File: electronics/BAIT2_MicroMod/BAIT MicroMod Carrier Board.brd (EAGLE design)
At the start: 95.2 x 94 mm, 108 parts, among them J1 microSD, J4 JST_6_PIN_VERTICAL, J5 QWIIC_RIGHT_ANGLE, U3 3.3V, U4 3.3V, U5 BQ27441-G1, X1 2.1mm DC, X2 BQ24074

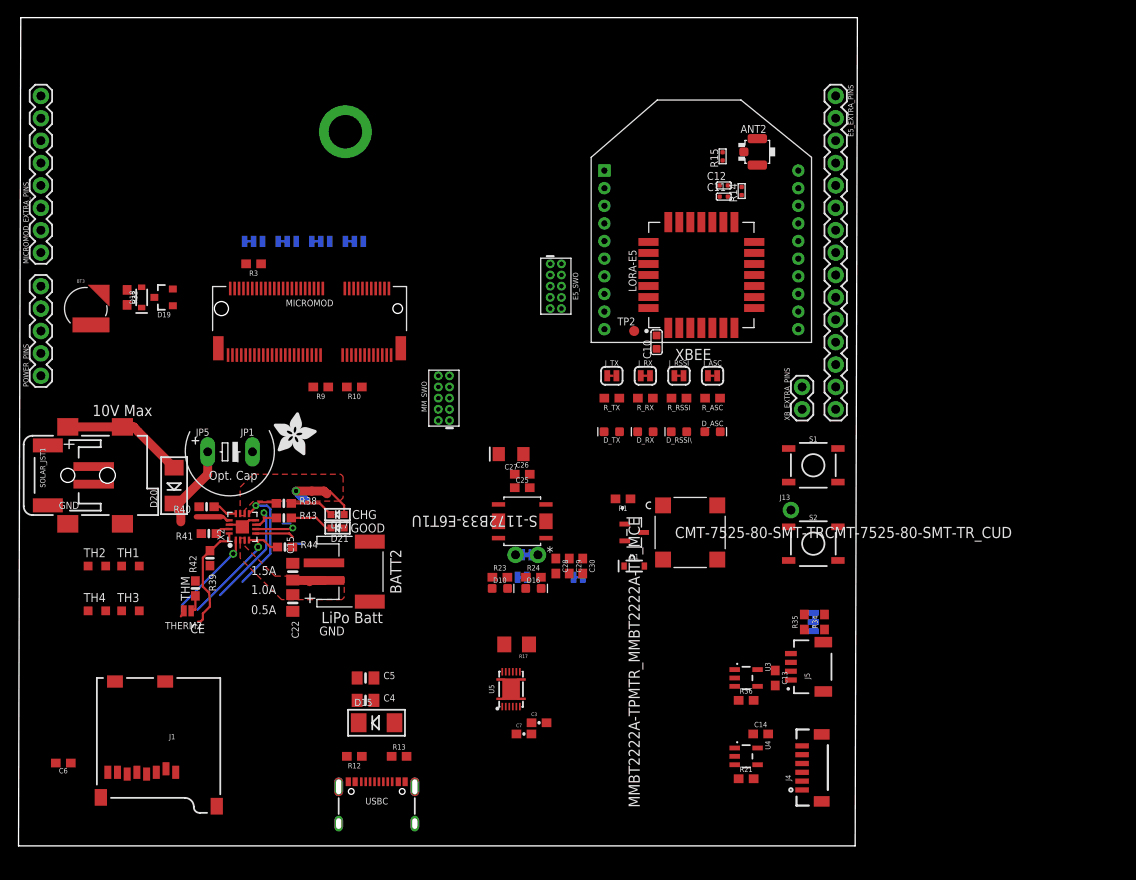
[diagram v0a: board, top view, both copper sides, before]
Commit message: Files for First Prototype production
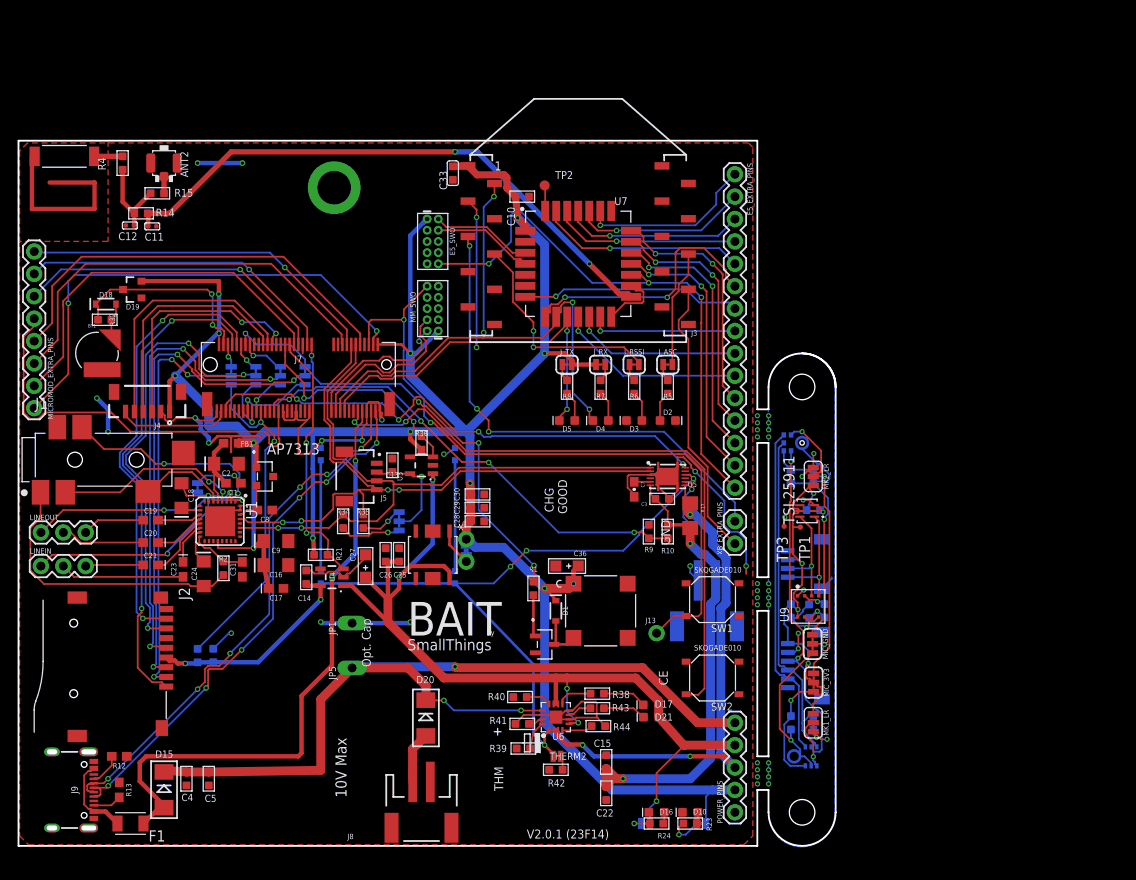
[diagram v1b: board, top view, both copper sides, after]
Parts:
- removed 3V3_LED2: (no value), SparkFun-Jumpers:SMT-JUMPER_2_NC_TRACE_SILK
- removed BATT2: JST 2PH, adafruit:JST-PH-2-SMT-RA
- removed BT3: ML414H, SparkFun-Batteries:ML414H_IV01E
- removed D_ASC, D_RSSI\, D_RX: GREEN, SparkFun-LED:LED-0603
- removed D_TX: RED, SparkFun-LED:LED-0603
- removed LORA-E5: LoRa-E5-HF, moudle-new:MOUDLE28P-1.25-12X12X2.5MM
- removed MICROMOD: MICROMOD-2222-C, SparkFun-MicroMod:M.2-CONNECTOR-E
- removed REG1: S-1172B33-E6T1U, Ablic:HSOP-6_FH006-A-P-SD-2.1_ABL
- removed R_ASC: 4.7k, SparkFun-Resistors:0603
- removed R_RSSI, R_RX, R_TX: 1k, SparkFun-Resistors:0603
- removed S1: Reset, SparkFun-Switches:TACTILE_SWITCH_SMD_5.2MM
- removed S2: BOOT, SparkFun-Switches:TACTILE_SWITCH_SMD_5.2MM
- removed SOLAR_JST1: (no value), SparkFun-Connectors:JST-2-SMD
- removed U$23: (no value), microbuilder:ADAFRUIT_5MM
- removed USBC: (no value), SparkFun-Connectors:USB-C-16P-2LAYER-PADS
- removed X1: 2.1mm DC, microbuilder:DCJACK_2MM_SMT
- removed X2: BQ24074, adafruit_power:QFN16_3MM
- removed XBEE: XBEE, adafruit:XBEE
- added 3V3_LED, GND_CON: (no value), SparkFun-Jumpers:SMT-JUMPER_2_NC_TRACE_SILK
- added ANT1: 0868AT43A0020EANT_0868AT43A0020E_JOT, 2023-01-04_20-35-52_Library:ANT_0868AT43A0020E_JOT
- added BT1: ML414H, SparkFun-Batteries:ML414H_IV01E
- added C1, C17, C19, C20, C21, C23, C31, C8: 2.2uF, SparkFun-Capacitors:0603-POLAR
- added C16, C2, C24, C9: 0.1uF, SparkFun-Capacitors:EIA3216
- added C18: 0.15uF, SparkFun-Capacitors:EIA3216
- added C32, C34, C35, C37, C38: 100nf, OPL_Capacitor:C0603
- added C33: 4.7uF, Discrete-new:C0603
- added C36: 10uf, OPL_Capacitor:AVX-A
- added C39: 220pF, Capacitor:CAPC1608X85
- added D2, D3, D4: GREEN, SparkFun-LED:LED-0603
- added D5: RED, SparkFun-LED:LED-0603
- added F1: 6V/2A, Circuit-Protection:FUSC3215X82N
- added FB1: 600Ω/1.8A, SparkFun-Coils:0603
- added J10: QWIIC_RIGHT_ANGLE, SM04B-SRSS-TB_LF__SN_:JST_SM04B-SRSS-TB(LF)(SN)
- added J15: SM06B-SRSS-TB(LF)(SN), SM06B-SRSS-TB_LF__SN_:JST_SM06B-SRSS-TB(LF)(SN)
- added J2: ST-TF-003A, ST-TF-003A:SUNTECH_ST-TF-003A
- added J3: (no value), SparkFun-RF:XBEE-SMD
- added J6: JST 2PH, adafruit:JST-PH-2-SMT-RA
- added J7: MICROMOD-2222-C, SparkFun-MicroMod:M.2-CONNECTOR-E
- added J8: (no value), SparkFun-Connectors:JST-2-SMD
- added J9: (no value), SparkFun-Connectors:USB-C-16P-2LAYER-PADS
- added LINEIN, LINEOUT: (no value), SparkFun-Connectors:1X03
- added MIC_3V3, MIC_GND: (no value), SparkFun-Jumpers:SMT-JUMPER_3_2-NC_TRACE_SILK
- added MK1: ICS-43432, Audio-Devices:ICS-43432
- added MK1_LR: MK1_LR, SparkFun-Jumpers:SMT-JUMPER_3_1-NC_TRACE_SILK
- added MK2: SPH0645LM4H-B, SPH0645LM4H-B:MIC_SPH0645LM4H-B
- added MK2_LR: MK2_LR, SparkFun-Jumpers:SMT-JUMPER_3_1-NC_TRACE_SILK
- added R11, R5: 4.7K, OPL_Resistor:R0603
- added R18: 100K, OPL_Resistor:R0603
- added R2: 2.2K, OPL_Resistor:R0603
- added R4: 0R, OPL_Resistor:R0603
- added R6, R7, R8: 1K 1/10W, OPL_Resistor:R0603
- added SW1, SW2: SKQGADE010, OPL_Switch:SW4-SMD-5.2X5.2X1.5MM
- added TP1, TP3: PTR1TP06R, testpad:TP06R
- added U1: SGTL5000-32, Freescale:QFN-32-5MM
- added U10: TSL25911, 2023-02-07_20-42-29_Library:SON-06-FN_2000X2400_AMS
- added U2: AP7313, 2022-08-05_10-01-44_Library:SOT-23_DIO
- added U6: BQ24074, adafruit_power:QFN16_3MM
- added U7: LoRa-E5-HF, moudle-new:MOUDLE28P-1.25-12X12X2.5MM
- added U8: S-1172B33-E6T1U, Ablic:HSOP-6_FH006-A-P-SD-2.1_ABL
- added U9: BOSCH_TOOLS_BME680BOSCH_TOOLS_BME680_0_0, Bosch Tools - BME680:BOSCH_TOOLS_BME680_0
- C10: value 4.7uF -> 4.7uf; device Discrete-new:C0603 -> OPL_Capacitor:C0603
- C13, C14, C28: value 1.0uF -> 1uf; device SparkFun-Capacitors:0603 -> OPL_Capacitor:C0603
- C15, C22, C4, C5: value 10uF -> 4.7uf; device microbuilder:0805-NO -> OPL_Capacitor:C0603
- C25, C30: value 0.22uF -> 220nf; device SparkFun-Capacitors:0603 -> OPL_Capacitor:C0603
- C26, C29, C6: value 0.1uF -> 100nf; device SparkFun-Capacitors:0603 -> OPL_Capacitor:C0603
- C27: value 10uF -> 10uf; device SparkFun-Capacitors:EIA3216 -> OPL_Capacitor:AVX-A
- C3: value 1.0uF -> 1uf; device SparkFun-Capacitors:0603-CAP -> OPL_Capacitor:C0603
- D17, D21: device microbuilder:CHIPLED_0603 -> SparkFun-LED:LED-0603
- J1: value microSD -> SJ-43516-SMT; device SparkFun-Connectors:MICRO-SD-SOCKET -> SnapEDA-Library:CUI_SJ-43516-SMT
- R1: value 180 -> 200K; device SparkFun-Resistors:0603 -> OPL_Resistor:R0603
- R10: value 20k -> 20K; device SparkFun-Resistors:0603 -> OPL_Resistor:R0603
- R14, R15: device Discrete-new:R0402 -> OPL_Resistor:R0603
- R21, R3, R36: value 100k -> 100K; device SparkFun-Resistors:0603 -> OPL_Resistor:R0603
- R23: value 1k -> 1K 1/10W; device SparkFun-Resistors:0603 -> OPL_Resistor:R0603
- R24: value 4.7k -> 4.7K; device SparkFun-Resistors:0603 -> OPL_Resistor:R0603
- R32: value 3.3k -> 3.3K; device SparkFun-Resistors:0603 -> OPL_Resistor:R0603
- R34, R35: value 2.2k -> 2.2K; device SparkFun-Resistors:0603 -> OPL_Resistor:R0603
- R38, R41, R42, R43, R44: value 10K -> 10K 1/10W; device microbuilder:0603-NO -> OPL_Resistor:R0603
- R39: device microbuilder:0603-NO -> OPL_Resistor:R0603
- R40: value 1K -> 1K 1/10W; device microbuilder:0603-NO -> OPL_Resistor:R0603
- R9: value 10k -> 10K 1/10W; device SparkFun-Resistors:0603 -> OPL_Resistor:R0603
- TH1, TH2, TH3, TH4: device varistor:CT/CN0603 -> NTCG163JX103DT1S:THERM_NTCG163JX103DT1S
- moved POWER_PINS 93.0 mm to (81.3, 3.81)
- moved J4 86.3 mm to (14.6, 50.5), turned to 180 degrees
- moved R14 68.2 mm to (13.9, 71.8), turned to 270 degrees
- moved C12 67.5 mm to (12.6, 70.4)
- moved ANT2 67.3 mm to (16.5, 77.5), turned to 90 degrees
- moved C11 64.9 mm to (15.2, 70.3), turned to 180 degrees
- moved R15 64.3 mm to (15.7, 74.0)
- moved R34 55.8 mm to (36.8, 36.8), turned to 0 degrees
- moved C14 54.5 mm to (32.6, 30.5), turned to 180 degrees
- moved R21 54.5 mm to (34.3, 33.0), turned to 270 degrees
- moved J5 51.7 mm to (40.6, 41.9), turned to 270 degrees
- moved R35 51.3 mm to (39.1, 36.8), turned to 0 degrees
- moved U4 51.2 mm to (35.6, 30.5), turned to 90 degrees
- moved C13 49.7 mm to (42.4, 43.2), turned to 180 degrees
- moved QWIIC_PWR 48.4 mm to (43.2, 36.8)
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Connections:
- removed net GND1: SOLAR_JST1.1, X1.2, X1.3
- removed net OUT: X2.5
- removed net PA15/SDA: LORA-E5.6
- removed net PB15/SCL: LORA-E5.5
- removed net RX2: MICROMOD.20
- removed net THERM: TH1.1, TH3.1, THERM2.2, X2.1
- removed net TX2: MICROMOD.22
- removed net V+1: REG1.6
- removed net VCC: XBEE.1
- new net 3V3_B: C34.1, C35.1, J10.2, J15.1, MIC_3V3.2, MK1_LR.1, MK2_LR.3, TP1.TP, U10.5, U9.8
- new net 3V3_ICS: C37.1, MIC_3V3.3, MK1.3
- new net 3V3_SPH: C38.1, C39.1, MIC_3V3.1, MK2.5
- new net AGND: C18.-, GND_CON.1, LINEIN.1, LINEOUT.1, U1.1, U1.3, U1.7
- new net GND_B: C32.2, C34.2, C35.2, J10.1, J10.S1, J10.S2, J15.2, J15.S1, J15.S2, MIC_GND.2, MK1_LR.3, MK2_LR.1, R18.1, TP3.TP, U10.3, U9.1, U9.5, U9.7
- new net GND_ICS: C37.2, MIC_GND.3, MK1.2, MK1.4
- new net GND_SPH: C38.2, C39.2, MIC_GND.1, MK2.3
- new net INT_B: U10.2
- new net N$11: ANT1.1, R4.2
- new net N$13: C19.-, LINEOUT.3
- new net N$14: C20.-, LINEOUT.2
- new net N$15: C21.-, LINEIN.3
- new net N$17: C23.-, LINEIN.2
- new net N$18: C19.+, U1.11
- new net N$20: C20.+, U1.12
- new net N$21: C21.+, U1.13
- new net N$22: C23.+, U1.14
- new net N$33: C24.-, J1.1, R2.2
- new net N$35: J1.3, U1.2
- new net N$36: F1.1, J9.VBUS1, J9.VBUS2
- new net N$38: C18.+, U1.10
- new net N$39: C31.+, R2.1, U1.16
- new net N$40: C24.+, U1.15
- new net N$41: C8.+, U1.30, U2.2
- new net N$46: C1.+, C2.+, FB1.2, U1.5
- new net N$54: C32.1, R11.2, U9.6
- new net N$55: R11.1, U9.2
- new net N$8: J1.2, U1.6
- new net SCK_B: J15.3, MK1.6, MK2.4
- new net SCL_B: J10.4, U10.1, U9.4
- new net SDA_B: J10.3, U10.6, U9.3
- new net SD_B: J15.4, MK1.7, MK2.6, R18.2
- new net SEL_MK1: MK1.1, MK1_LR.2
- new net SEL_MK2: MK2.2, MK2_LR.2
- new net USB_VIN: D15.A, F1.2, J7.9
- new net WS_B: J15.5, MK1.5, MK2.1
- net !BOOT!: now also J7.11, SW2.2; no longer MICROMOD.11, S2.3, S2.4
- net !CE: now also U6.4; no longer X2.4
- net !CHG: now also U6.9; no longer X2.9
- net !PGOOD: now also U6.7; no longer X2.7
- net !RESET!: now also J7.6, SW1.2; no longer MICROMOD.6, S1.3, S1.4
- net 3.3V: now also 3V3_LED.2, C16.+, C17.+, C33.2, C36.+, C9.+, FB1.1, J3.1, J7.2, J7.74, J_RX.1, U1.20, U2.1, U7.1; no longer 3V3_LED2.2, J_RX.2, LORA-E5.1, MICROMOD.2, MICROMOD.74
- net 3.3V_EN: now also J7.4; no longer MICROMOD.4
- net 3.3V_LP: now also J2.4; no longer J1.VCC
- net A0: now also J7.34; no longer MICROMOD.34
- net A1: now also J7.38; no longer MICROMOD.38
- net ASC: now also J3.15; no longer XBEE.15
- net CLK/SCK: now also J2.5, JP_SCK.2; no longer J1.SCLK, JP_SCK.3
- net CMD/CIPO: now also J2.3, JP_CIPO.2; no longer J1.DI/CMD, JP_CIPO.3
- net D0: now also J7.10; no longer MICROMOD.10
- net D1: now also J7.18; no longer MICROMOD.18
- net DAT0/COPI: now also J2.7, JP_COPI.2; no longer J1.DO/DAT0, JP_COPI.3
- net DAT3/!CS!: now also J2.2, JP_CS.2; no longer J1.CS/DAT3, JP_CS.3
- net GND: now also BT1.-, C1.-, C16.-, C17.-, C2.-, C31.-, C33.1, C36.-, C8.-, C9.-, D2.C, D3.C, GND_CON.2, J2.6, J2.G1, J2.G2, J2.G3, J2.G4, J3.10, J6.2, J7.1, J7.33, J7.36, J7.39, J7.45, J7.7, J7.75, J8.1, J9.GND, J9.GND2, SW1.4, SW2.4, U1.31, U1.32, U1.PAD, U2.3, U6.14, U6.6, U6.8, U6.THERMAL, U7.14, U7.16, U7.2, U7.22, U8.2, U8.5; no longer BATT2.2, BT3.-, D_ASC.C, D_RSSI\.C, J1.CD1, J1.GND, J1.GND1, J1.GND3, LORA-E5.14, LORA-E5.16, LORA-E5.2, LORA-E5.22, MICROMOD.1, MICROMOD.33, MICROMOD.36, MICROMOD.39, MICROMOD.45, MICROMOD.7, MICROMOD.75, REG1.2, REG1.5, S1.1, S1.2, S2.1, S2.2, USBC.GND, USBC.GND2, X2.14, X2.6, X2.8, X2.THERMAL, XBEE.10
- net GPOUT: now also J7.71
- net HEADER_!CS!: now also J7.40; no longer MICROMOD.40
- net I2C_!INT!: now also J7.16; no longer MICROMOD.16
- net I2C_SCL: now also J7.14, U1.29; no longer MICROMOD.14
- net I2C_SDA: now also J7.12, U1.27; no longer MICROMOD.12
- net I2S_SCK: now also J7.50; no longer MICROMOD.50
- net I2S_SD: now also J7.54; no longer MICROMOD.54
- net I2S_WS: now also J7.52; no longer MICROMOD.52
- net ILIM: now also U6.12; no longer X2.12
- net ISET: now also U6.16; no longer X2.16
- net ITERM: now also U6.15; no longer X2.15
- net LR_SEL: now also J7.73; no longer MICROMOD.73
- net N$16: now also 3V3_LED.1; no longer 3V3_LED2.1
- net N$19: now also U7.28; no longer LORA-E5.28
- net N$23: now also BT1.+; no longer BT3.+
- net N$25: now also R5.2; no longer R_ASC.2
- net N$28: now also R4.1
- net N$3: now also J_RX.2, R7.2; no longer J_RX.1, R_RX.2
- net N$30: now also J8.2; no longer SOLAR_JST1.2, X1.1, X1.1'
- net N$34: now also D2.A, R5.1; no longer D_ASC.A, R_ASC.1
- net N$4: now also J9.A5; no longer USBC.A5
- net N$42: now also R6.2; no longer R_RSSI.2
- net N$43: now also D3.A, R6.1; no longer D_RSSI\.A, R_RSSI.1
- net N$44: now also R8.2; no longer R_TX.2
- net N$45: now also D5.A, R8.1; no longer D_TX.A, R_TX.1
- net N$48: now also J1.4, U1.4; no longer D15.A, USBC.VBUS1, USBC.VBUS2
- net N$5: now also J9.B5; no longer USBC.B5
- net N$6: now also U8.1; no longer REG1.1
- net N$9: now also D4.A, R7.1; no longer D_RX.A, R_RX.1
- net PA0/D0: now also U7.23; no longer LORA-E5.23
- net PA10/MOSI: now also U7.27; no longer LORA-E5.27
- net PA13/SWDIO: now also U7.3; no longer LORA-E5.3
- net PA14/SWCLK: now also U7.4; no longer LORA-E5.4
- net PA2/TX2: now also U7.19; no longer LORA-E5.19
- net PA3/RX2: now also E5_EXTRA_PINS.14, U7.18; no longer E5_EXTRA_PINS.12, LORA-E5.18
- net PA9/D9: now also E5_EXTRA_PINS.11, U7.21; no longer E5_EXTRA_PINS.15, LORA-E5.21
- net PB10/D10: now also E5_EXTRA_PINS.12, U7.20; no longer E5_EXTRA_PINS.14, LORA-E5.20
- net PB13/BOOT/SCK: now also U7.24; no longer LORA-E5.24
- net PB14/MISO: now also U7.26; no longer LORA-E5.26
- net PB3/A3: now also U7.8; no longer LORA-E5.8
- net PB4/A4: now also U7.7; no longer LORA-E5.7
- net PB5/LED: now also E5_EXTRA_PINS.10, U7.11; no longer E5_EXTRA_PINS.8, LORA-E5.11
- net PB9/NSS: now also U7.25; no longer LORA-E5.25
- net PC0/RX1: now also E5_EXTRA_PINS.8, U7.13; no longer E5_EXTRA_PINS.10, LORA-E5.13
- net PC1/TX1: now also U7.12; no longer LORA-E5.12
- net PERIPHERAL_PWR_CTRL: now also J7.42; no longer MICROMOD.42
- net PWM0: now also J7.32; no longer MICROMOD.32
- net PWM1: now also J7.47; no longer MICROMOD.47
- net QWIIC_PWR_CTRL: now also J7.44; no longer MICROMOD.44
- net RF: now also U7.15; no longer LORA-E5.15
- net RSSI: now also J3.6; no longer XBEE.6
- net RST: now also E5_EXTRA_PINS.15, U7.17; no longer E5_EXTRA_PINS.11, LORA-E5.17
- net RTC_3V: now also J7.72; no longer MICROMOD.72
- net RX: now also D4.C, J3.2, J7.19, U7.9; no longer D_RX.C, LORA-E5.9, MICROMOD.19, XBEE.2
- net SD_!CS!: now also J7.55; no longer MICROMOD.55
- net SD_CLK: now also J7.60, JP_SCK.3; no longer JP_SCK.2, MICROMOD.60
- net SD_CMD: now also J7.62, JP_CIPO.3; no longer JP_CIPO.2, MICROMOD.62
- net SD_DATA0: now also J7.64, JP_COPI.3; no longer JP_COPI.2, MICROMOD.64
- net SD_DATA1: now also J2.8, J7.66; no longer J1.DAT1, MICROMOD.66
- net SD_DATA2: now also J2.1, J7.68; no longer J1.DAT2, MICROMOD.68
- net SD_DATA3: now also J7.70, JP_CS.3; no longer JP_CS.2, MICROMOD.70
- net SPI_CIPO: now also J7.61; no longer MICROMOD.61
- net SPI_COPI: now also J7.59; no longer MICROMOD.59
- net SPI_SCK: now also J7.57; no longer MICROMOD.57
- net SWDCK: now also J7.21; no longer MICROMOD.21
- net SWDIO: now also J7.23; no longer MICROMOD.23
- net TS: now also TH1.1, TH3.1, THERM2.2, U6.1
- net TX: now also D5.C, J3.3, J7.17, U7.10; no longer D_TX.C, LORA-E5.10, MICROMOD.17, XBEE.3
- net USB_D+: now also J7.3, J9.A6, J9.B6; no longer MICROMOD.3, USBC.A6, USBC.B6
- net USB_D-: now also J7.5, J9.A7, J9.B7; no longer MICROMOD.5, USBC.A7, USBC.B7
- net V+: now also U6.10, U6.11, U6.5, U8.6; no longer X2.10, X2.11
- net VBUS: now also U6.13; no longer X2.13
- net VIN: now also J6.1; no longer BATT2.1, MICROMOD.9
- net VIN/3: now also J7.49; no longer MICROMOD.49
- net V_BATT: now also U6.2, U6.3; no longer X2.2, X2.3
- net XB_ON: now also J3.13; no longer XBEE.13
- net XB_RST: now also J3.5; no longer XBEE.5
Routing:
- net 3.3V: track 0.00 -> 271.8 mm, vias 0 -> 13
- net GND: track 7.68 -> 153.4 mm, vias 1 -> 17
- net V+: track 10.4 -> 109.5 mm, vias 1 -> 5
- net VBUS: track 13.9 -> 101.7 mm, vias 0 -> 3
- net !RESET!: track 0.00 -> 79.7 mm, vias 0 -> 2
- net TS: track 0.00 -> 74.5 mm, vias 0 -> 4
- net I2C_SCL: track 0.00 -> 74.4 mm, vias 0 -> 4
- net I2C_SDA: track 0.00 -> 74.1 mm, vias 0 -> 2
- net !BOOT!: track 0.00 -> 72.1 mm, vias 0 -> 2
- net USB_VIN: track 0.00 -> 69.8 mm, vias 0 -> 2
- net RF: track 0.00 -> 66.0 mm, vias 0 -> 2
- net RX: track 0.00 -> 66.0 mm, vias 0 -> 4
- net RST: track 0.00 -> 63.7 mm, vias 0 -> 3
- net USB_D+: track 0.00 -> 61.5 mm, vias 0 -> 6
- net TX: track 0.00 -> 61.0 mm, vias 0 -> 4
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- added copper zone on layer 1, net CUTOUT
- added copper zone on layer 1, net GND
- added copper zone on layer 16, net GND_B
- removed copper zone on layer 1, net OUT
- removed copper zone on layer 1, net VLIPO
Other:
- board size 95.2 x 94 mm -> 92.7 x 80 mm
- board text added: "50 ohm impedance control on the RF line from its origin on the WIO-E5 chip through to ANT1 and ANT2"
- board text added: "BAIT"
- board text added: "SmallThings"
- board text added: "V2.0.1 (23F14)"
- board text added: "by"
- board text removed: "0.5A"
- board text removed: "1.0A"
- board text removed: "1.5A"
- board text removed: "LiPo"
- board text removed: "LiPo Batt"
- board text removed: "Solar/DC In is 10V Max"
- board text removed: "Use any 3.7/4.2V LiPoly/LiIon"
